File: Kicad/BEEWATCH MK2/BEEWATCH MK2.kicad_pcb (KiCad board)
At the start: 4 copper layers, 40.3 x 39.7 mm, 119 parts, among them J1 USB_C_Receptacle_USB2.0_16P, J3 Conn_02x06_Odd_Even, Q1 DMG6968U, Q2 DMG6968U, Q3 DMP1045U-7, Q4 DMG6968U, Q5 BSS138, Q6 BSS138, Q7 BSS138, Q8 DMP1045U-7, Q9 DMG6968U, SW1 TK-074-4, SW2 TK-074-4, U1 ESP32-S3FH4R2, U2 LTC3549EDCB#TRMPBF, U3 MPU-6050, U4 MCP73832-2-OT, U5 ME6217C33M5G, U7 RYS8830, U8 S-1206B18-M3T1G, Y1 40MHz, Y2 32.768KHz

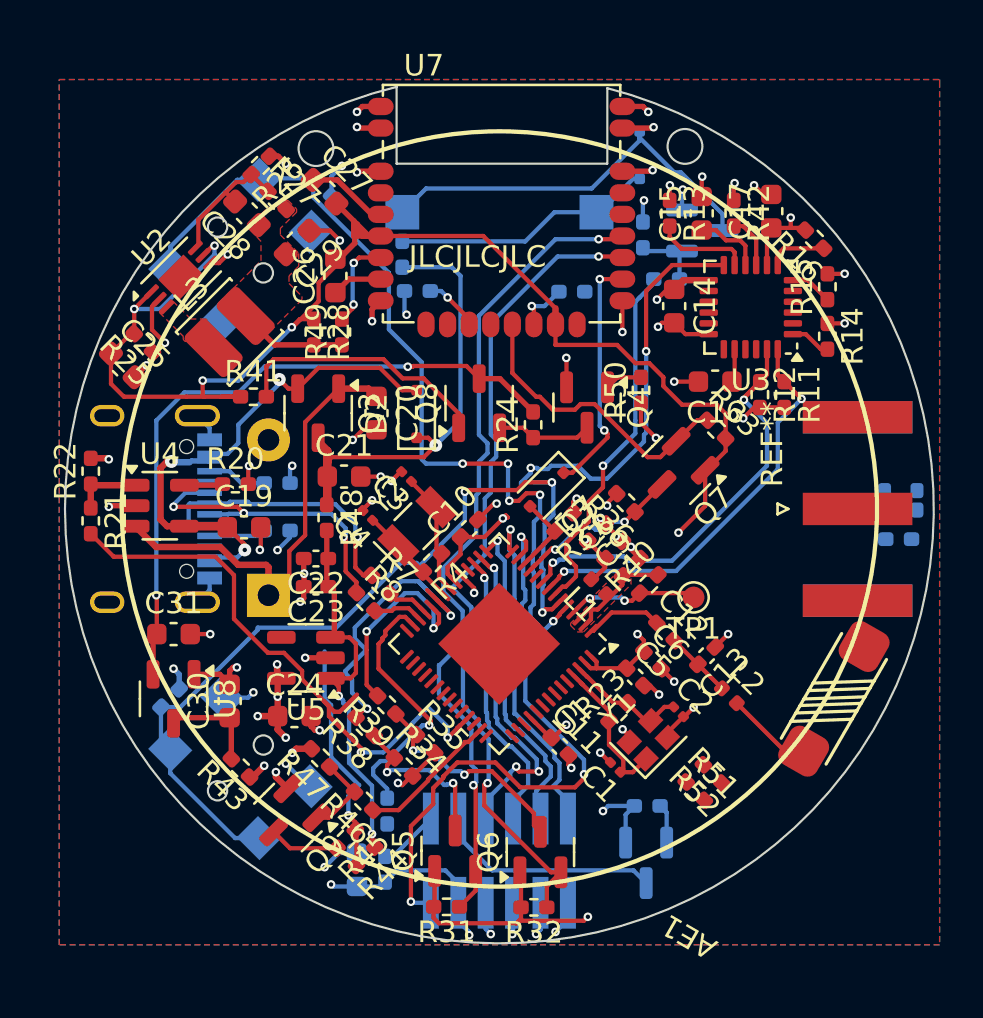
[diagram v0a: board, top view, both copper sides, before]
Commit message: Layout almost completed
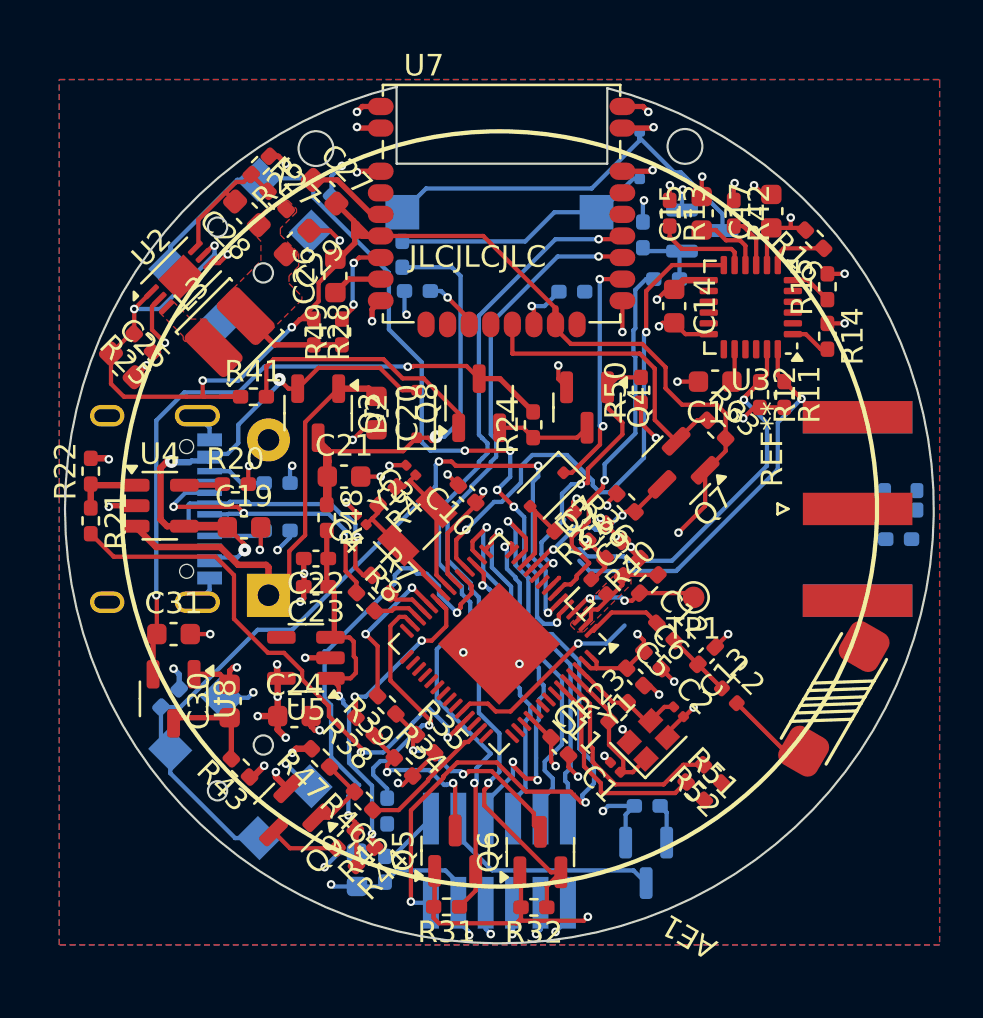
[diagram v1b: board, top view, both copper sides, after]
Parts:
- moved R4 3.74 mm to (144.8, 104.4)
- moved C10 1.60 mm to (148.5, 104.3), turned to 135 degrees
- moved C4 0.36 mm to (143.6, 105.5)
- moved C3 0.36 mm to (145.9, 103.2)
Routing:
- net /ESP32/GPS_EN: track 1.74 -> 13.6 mm, vias 0 -> 2
- net /ESP32/BAT_VSENSE: track 12.0 -> 22.2 mm
- net Net-(U1-GPIO46): track 0.00 -> 10.2 mm
- net Net-(U1-GPIO45): track 0.00 -> 9.80 mm
- net /ESP32/LED1: track 0.00 -> 9.50 mm, vias 0 -> 1
- net /ACCELEROMETER/MPU_INT: track 18.5 -> 25.8 mm
- net /ESP32/GPS_TXD: track 14.5 -> 8.44 mm
- net /Display/TFT_SDI: track 15.4 -> 19.7 mm
- net /Display/TFT_RST: track 28.5 -> 32.5 mm
- net /Display/TFT_CS: track 15.9 -> 18.5 mm
- net /ESP32/GPS_RXD: track 9.48 -> 7.38 mm
- net /Battery&BMS/CHG_ST: track 27.8 -> 25.8 mm
- net /ACCELEROMETER/MPU_SCL: track 20.9 -> 18.9 mm, vias 2 -> 1
- net /ESP32/IO0: track 39.9 -> 38.3 mm
- net /ESP32/XTAL_32K_N: track 4.80 -> 6.02 mm
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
